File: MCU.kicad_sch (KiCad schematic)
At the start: 101 parts, among them J301 I2C1, J302 I2C4, U301 MICROCONTROLLER, X301 25MHz 8pF

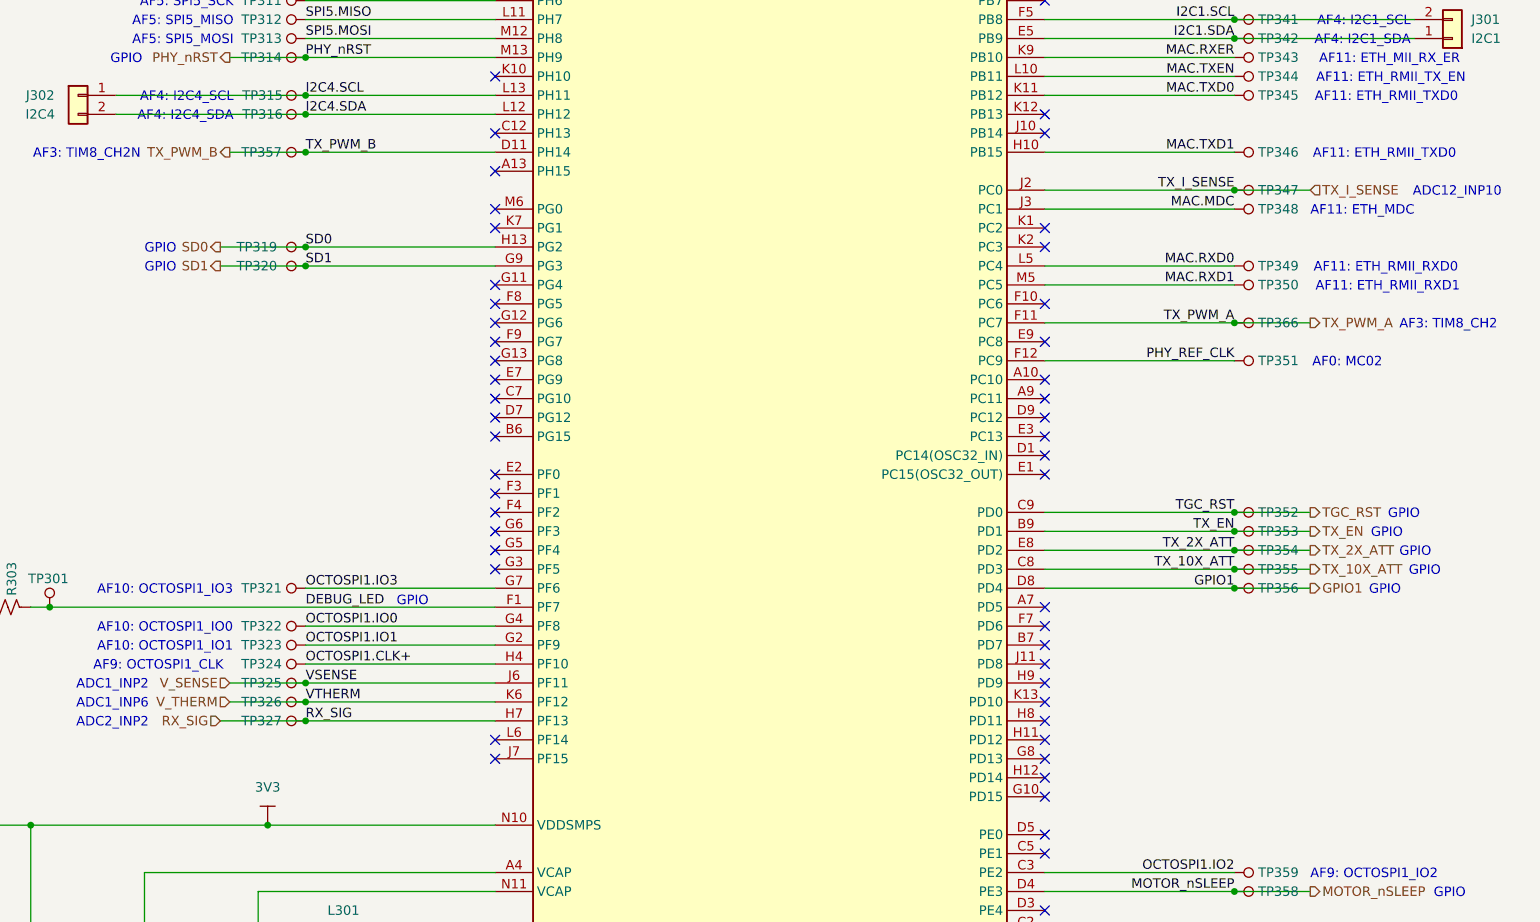
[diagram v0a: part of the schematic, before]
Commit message: starting to incorporate todos
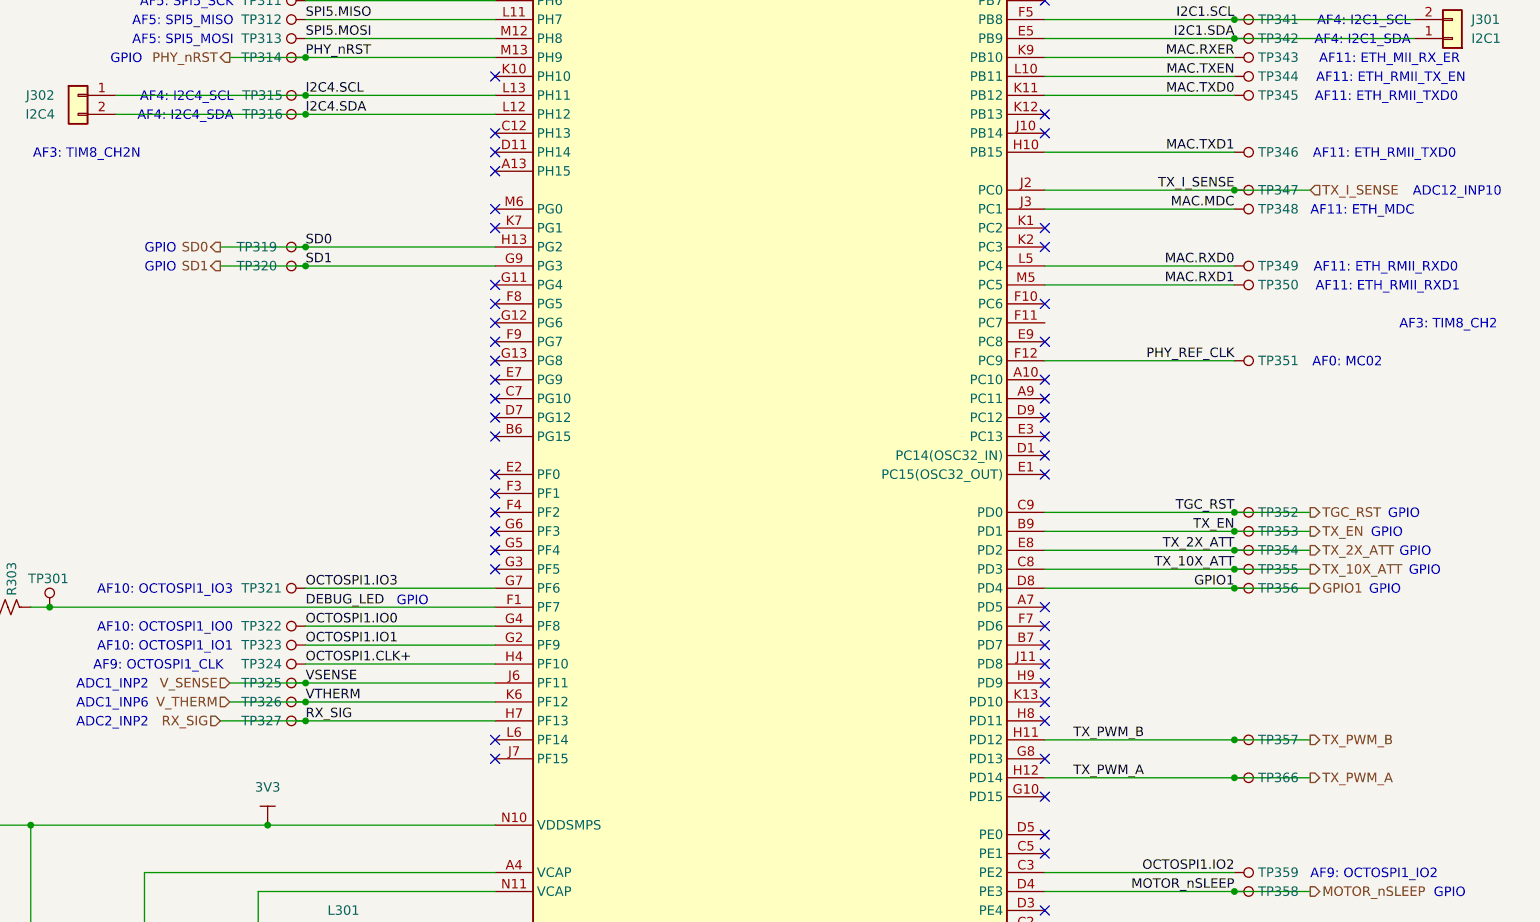
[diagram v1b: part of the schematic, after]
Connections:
- net TX_PWM_A: now also U301.H12 (PD14); no longer U301.F11 (PC7)
- net TX_PWM_B: now also U301.H11 (PD12); no longer U301.D11 (PH14)
- no-connect marks 69 -> 68
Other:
- moved on the sheet: TP357, TP366
